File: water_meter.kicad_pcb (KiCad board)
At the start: 4 copper layers, 94 x 64 mm, 50 parts, among them J1 2464, J2 Conn_01x02_Male, J3 Conn_01x06_Male, J4 USB_Micro-10118193-0001LF, J5 Conn_01x02_Male, J8 Conn_01x02_Male, U1 RT9080-33GJ5, U2 ESP32-S3-WROOM-1, U3 ALT025-10E, U4 SLG46826G, U5 PCF8563TS, Y1 32.768kHz (ESR < 70 kΩ), Y2 Crystal

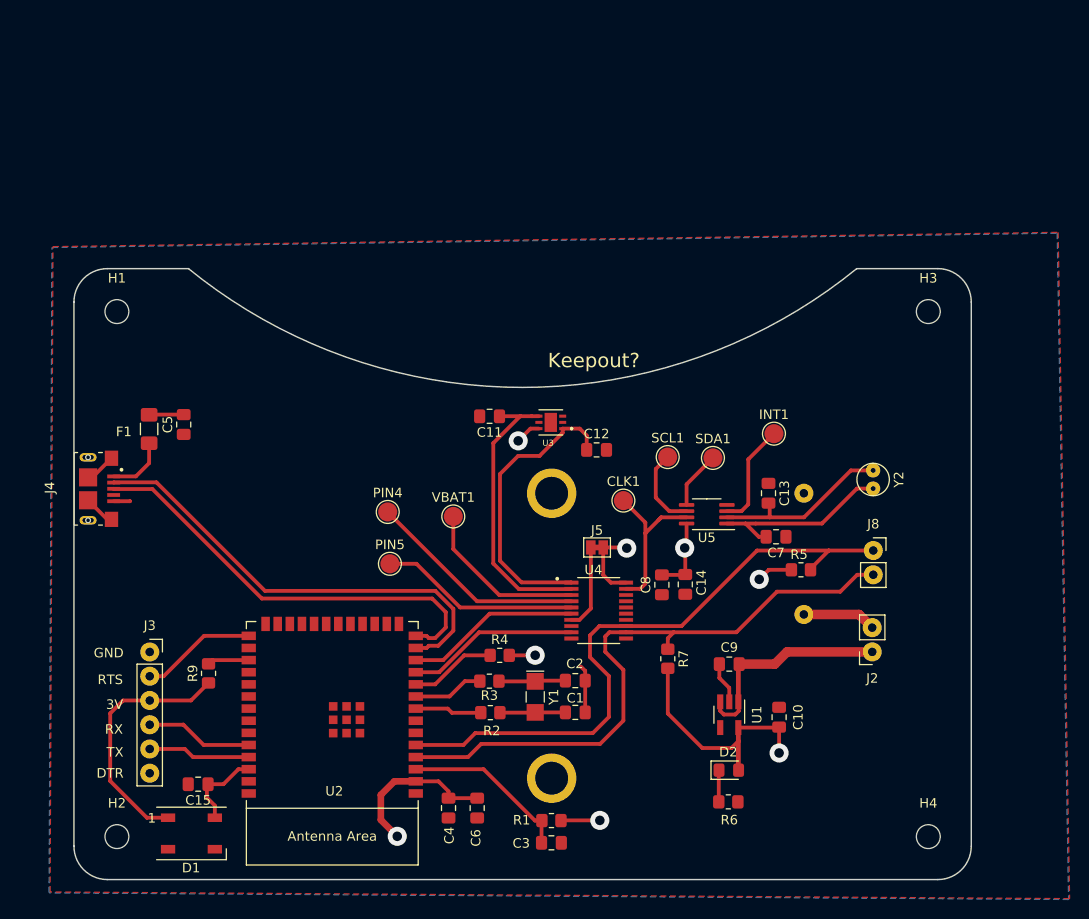
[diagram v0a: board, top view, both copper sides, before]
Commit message: V2
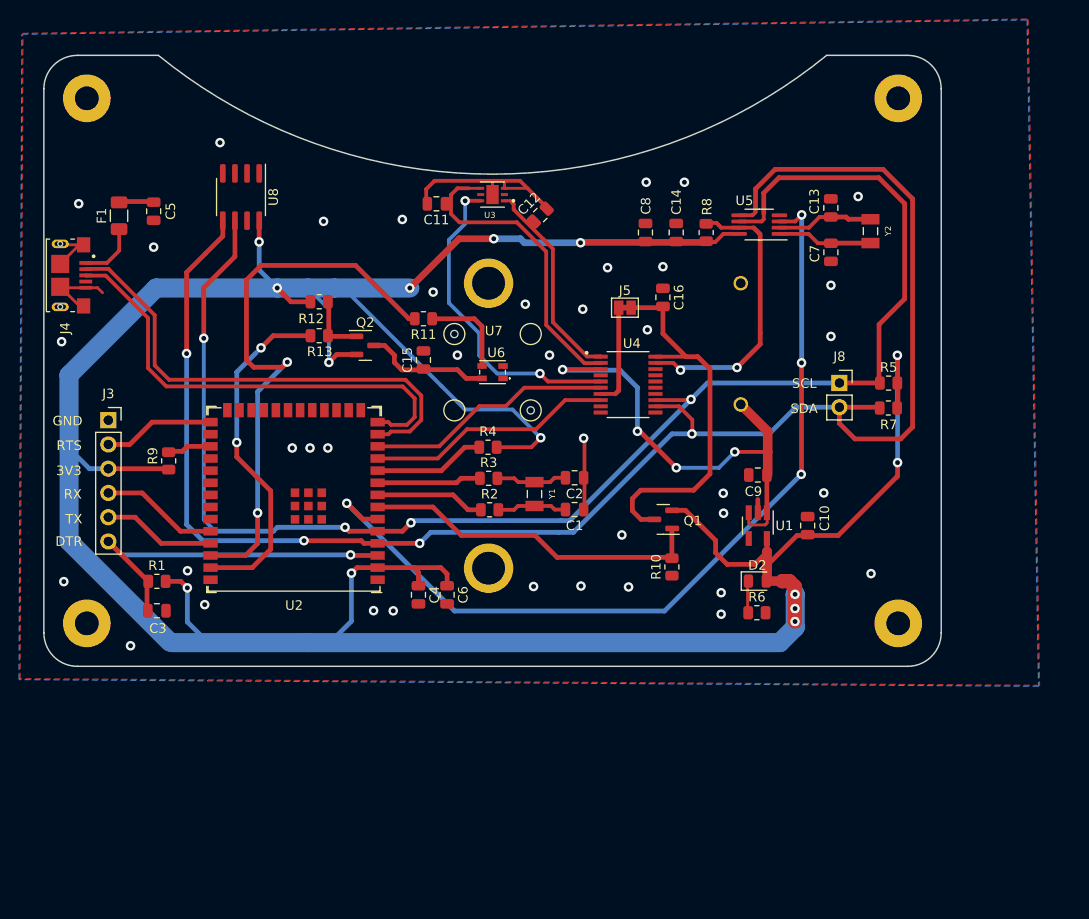
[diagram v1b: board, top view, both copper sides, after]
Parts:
- removed CLK1, INT1, PIN4, PIN5, SCL1, SDA1, VBAT1: TestPoint, TestPoint:TestPoint_Pad_D2.0mm
- removed D1: WS2812B, LED_SMD:LED_WS2812B_PLCC4_5.0x5.0mm_P3.2mm
- removed J2: Conn_01x02_Male, Connector_PinSocket_2.54mm:PinSocket_1x02_P2.54mm_Vertical
- added C16: 0.1uF, Capacitor_SMD:C_0805_2012Metric, F.Cu at (175.2, 109.0)
- added Q1: BSS84, Package_TO_SOT_SMD:SOT-23, F.Cu at (175.2, 132.3)
- added Q2: BSS84, Package_TO_SOT_SMD:SOT-23, F.Cu at (144.0, 114.0)
- added R10: 100k, Resistor_SMD:R_0805_2012Metric, F.Cu at (176.1, 137.2)
- added R11: 500R, Resistor_SMD:R_0805_2012Metric, F.Cu at (150.1, 111.3)
- added R12: 500R, Resistor_SMD:R_0805_2012Metric, F.Cu at (139.2, 109.5)
- added R13: 500R, Resistor_SMD:R_0805_2012Metric, F.Cu at (139.2, 113.0)
- added R8: 100k, Resistor_SMD:R_0805_2012Metric, F.Cu at (179.7, 102.2)
- added U6: IN-PI22TAT5R5G5B, Nabil:INPI22TAT5R5G5B, F.Cu at (157.3, 116.8)
- added U7: 10413_lens, Nabil:10414_Lens, F.Cu at (157.3, 116.8)
- added U8: FM24C64C, Package_SO:SOIC-8_3.9x4.9mm_P1.27mm, F.Cu at (131.0, 98.5)
- C1, C10, C11, C12, C13, C14, C15, C2, C3, C4, C6, C7, C8, C9: footprint Capacitor_SMD:C_0805_2012Metric_Pad1.18x1.45mm_HandSolder -> Capacitor_SMD:C_0805_2012Metric
- C5: value 10uF/25V(20%) -> 10uF; footprint Capacitor_SMD:C_0805_2012Metric_Pad1.18x1.45mm_HandSolder -> Capacitor_SMD:C_0805_2012Metric
- D2: footprint LED_SMD:LED_0805_2012Metric_Pad1.15x1.40mm_HandSolder -> LED_SMD:LED_0805_2012Metric
- F1: footprint Fuse:Fuse_1206_3216Metric_Pad1.42x1.75mm_HandSolder -> Fuse:Fuse_1206_3216Metric
- H1, H2, H3, H4: footprint MountingHole:MountingHole_2.5mm -> MountingHole:MountingHole_2.5mm_Pad
- R1: value 10k(1%) -> 10k; footprint Resistor_SMD:R_0805_2012Metric_Pad1.20x1.40mm_HandSolder -> Resistor_SMD:R_0805_2012Metric
- R2, R3, R4, R5, R6, R7, R9: footprint Resistor_SMD:R_0805_2012Metric_Pad1.20x1.40mm_HandSolder -> Resistor_SMD:R_0805_2012Metric
- U2: footprint Espressif:ESP32-S3-WROOM-1 -> Espressif:ESP32-S3-WROOM-1U
- Y1: value 32.768kHz (ESR < 70 kΩ) -> ABS07-32.768KHZ-T; footprint Crystal:Crystal_SMD_G8-2Pin_3.2x1.5mm_HandSoldering -> Nabil:XTAL_ABS07-32.768KHZ-T
- Y2: value Crystal -> ABS07-32.768KHZ-T; footprint Crystal:Crystal_C38-LF_D3.0mm_L8.0mm_Vertical -> Nabil:XTAL_ABS07-32.768KHZ-T
- moved C15 50.3 mm to (150.1, 115.6), turned to 90 degrees
- moved R1 48.3 mm to (122.2, 138.8)
- moved C3 47.9 mm to (122.2, 141.8)
- moved C8 36.9 mm to (173.4, 102.2), turned to -90 degrees
- moved C14 36.9 mm to (176.6, 102.2), turned to -90 degrees
- moved R7 35.0 mm to (198.8, 120.6), turned to 0 degrees
- moved U5 30.8 mm to (185.3, 101.4)
- moved C13 30.6 mm to (192.8, 99.6)
- moved C7 30.3 mm to (192.8, 104.3), turned to 90 degrees
- moved C12 25.3 mm to (162.3, 100.4), turned to 45 degrees
- moved J5 25.3 mm to (171.2, 110.1)
- moved Y2 25.1 mm to (196.9, 102.1)
- moved J3 24.7 mm to (117.1, 121.9)
- moved U3 24.6 mm to (157.3, 98.2)
- moved U4 23.9 mm to (171.6, 118.2)
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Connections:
- C15 pad 1: /LED_PIN0 -> Net-(Q2-Pad3)
- J1 pad 1: Net-(J2-Pad2) -> /VBATT
- J5 pad 2: +3V3 -> /SLG_PWR
- U2 pad 39: unconnected-(U2-Pad39) -> /LED_PWR
- U2 pad 6: unconnected-(U2-Pad6) -> /RTC_INT
- U2 pad 7: unconnected-(U2-Pad7) -> /SLG_PWR_GPIO
- U3 pad 6: +3V3 -> /MAG_PWR
- U4 pad 20: +3V3 -> /SLG_PWR
- U4 pad 4: Net-(U4-Pad4) -> unconnected-(U4-Pad4)
- U4 pad 5: Net-(U4-Pad5) -> /MAG_PWR
- U4 pad 8: unconnected-(U4-Pad8) -> /SLG_INT2
- U4 pad 9: /SLG_INT2 -> unconnected-(U4-Pad9)
- U5 pad 3: Net-(U5-Pad3) -> /RTC_INT
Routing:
- net +3V3: track 97.8 -> 341.0 mm, vias 8 -> 14
- net /SDA: track 71.8 -> 175.9 mm, vias 0 -> 4
- net /RTC_INT: track 0.00 -> 92.0 mm, vias 0 -> 4
- net /SCL: track 75.6 -> 156.3 mm, vias 0 -> 4
- net /LED_PIN0: track 8.82 -> 59.4 mm, vias 0 -> 2
- net /SLG_PWR: track 0.00 -> 39.9 mm
- net /LED_PWR: track 0.00 -> 36.3 mm, vias 0 -> 2
- net /SLG_PWR_GPIO: track 0.00 -> 36.1 mm
- net /MAG_PWR: track 0.00 -> 33.7 mm, vias 0 -> 2
- net GND: track 17.7 -> 42.6 mm, vias 0 -> 39
- net Net-(U4-Pad4): track 23.1 -> 0.00 mm
- net Net-(U4-Pad5): track 20.9 -> 0.00 mm
- net /EN: track 17.8 -> 37.8 mm, vias 0 -> 1
- net Net-(Q2-Pad3): track 0.00 -> 13.2 mm
- net /M_CLK: track 17.3 -> 30.1 mm, vias 0 -> 2
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- added copper zone on B.Cu, net GND
- removed copper zone on B.Cu, net +3V3
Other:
- board text added: "3V3"
- board text added: "SCL"
- board text added: "SDA"
- board text removed: "3V"
- board text removed: "Keepout?"
